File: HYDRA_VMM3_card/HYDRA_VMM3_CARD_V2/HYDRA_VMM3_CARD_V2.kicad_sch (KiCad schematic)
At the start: 17 parts, among them J1 ME1014010101011

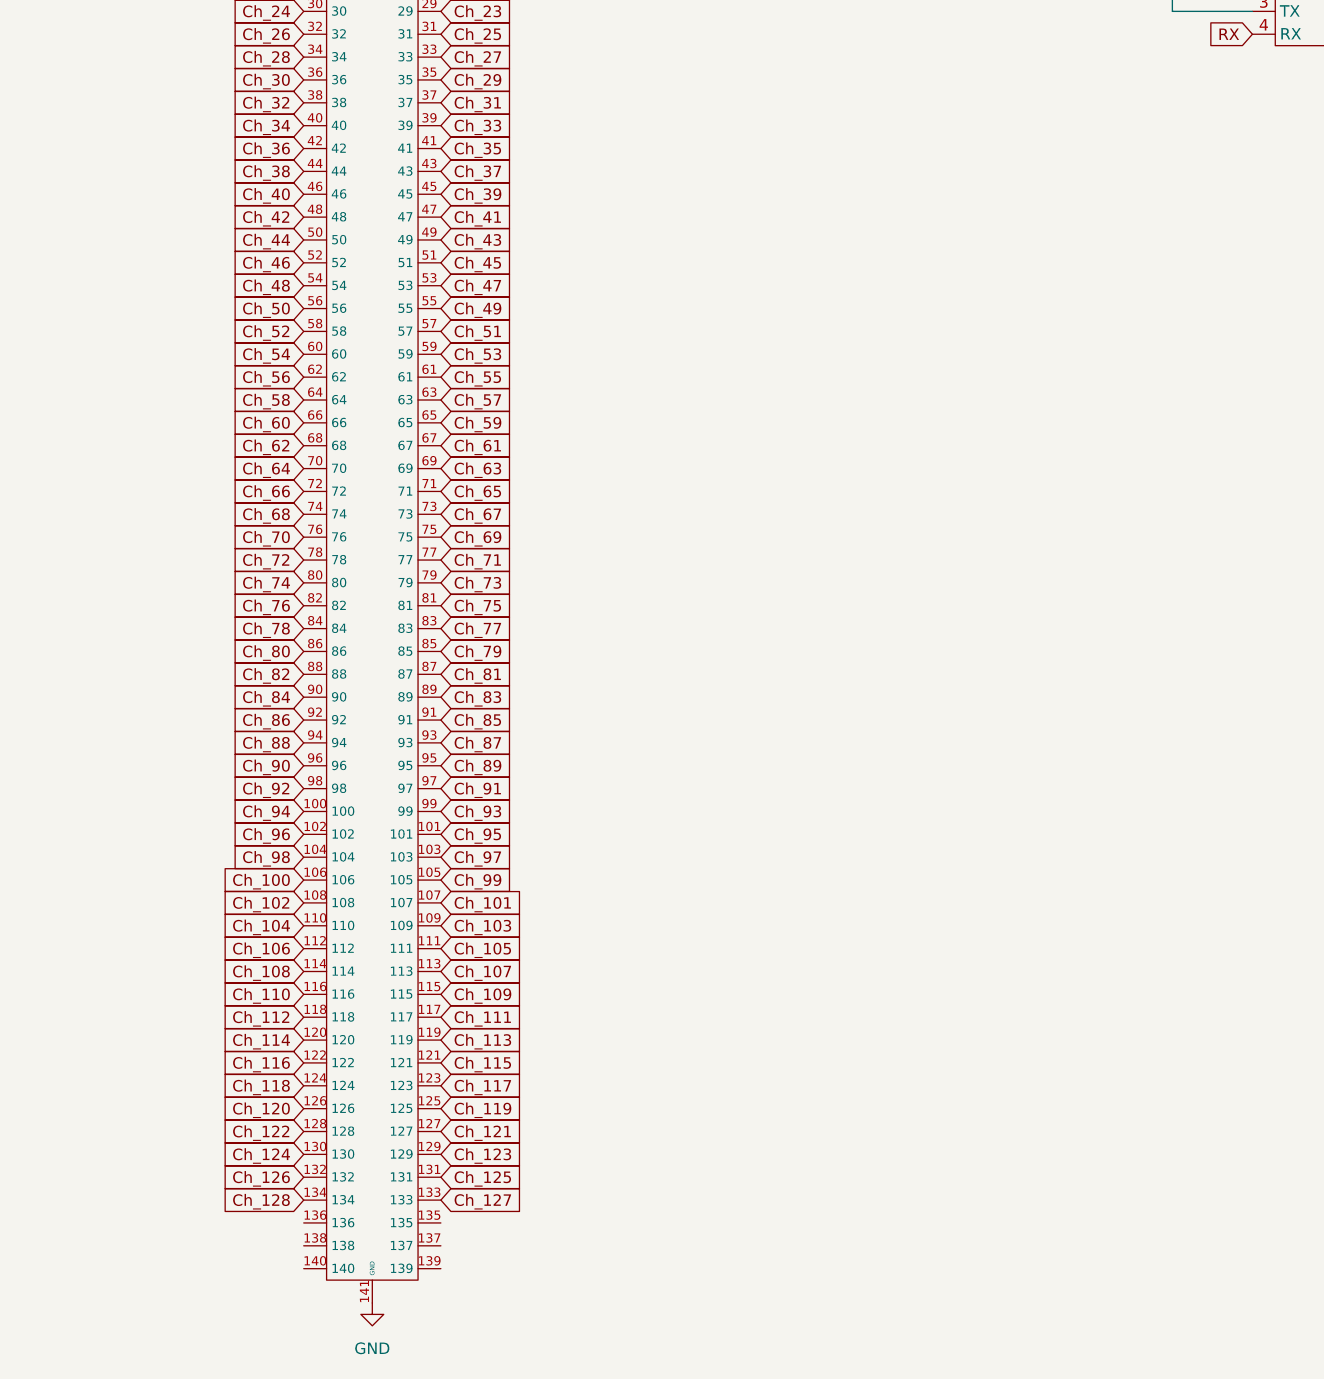
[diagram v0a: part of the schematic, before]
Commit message: .
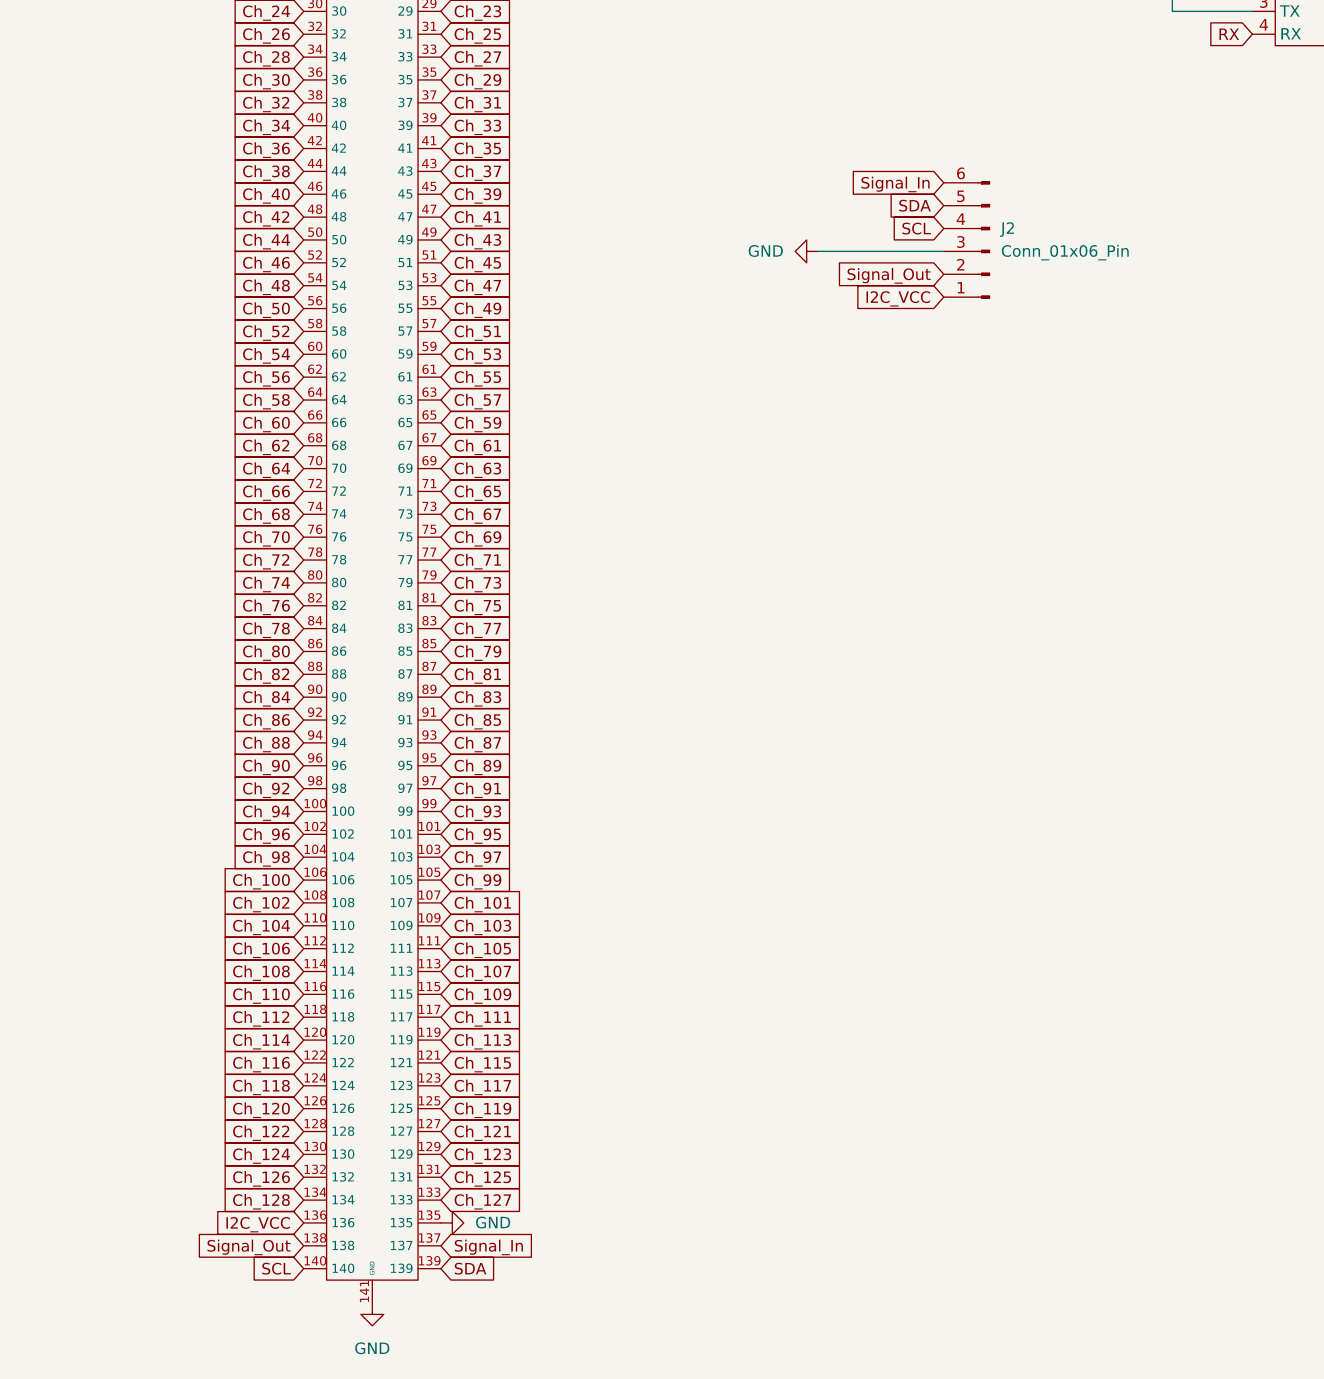
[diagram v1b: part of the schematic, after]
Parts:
- added J2: Conn_01x06_Pin, Connector_PinHeader_1.00mm:PinHeader_1x06_P1.00mm_Horizontal, symbol Connector:Conn_01x06_Pin
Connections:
- net GND: now also U1.135, J2.3 (Pin_3)
- net I2C_VCC: now reaches U1.136
- net I2C_VCC: now also J2.1 (Pin_1)
- net Signal_In: now reaches U1.137
- net Signal_In: now also J2.6 (Pin_6)
- net Signal_Out: now reaches U1.138
- net Signal_Out: now also J2.2 (Pin_2)
- net SDA: now reaches U1.139
- net SDA: now also J2.5 (Pin_5)
- net SCL: now reaches U1.140
- net SCL: now also J2.4 (Pin_4)

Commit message: .
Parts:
- removed J2: Conn_01x06_Pin, Connector_PinHeader_1.00mm:PinHeader_1x06_P1.00mm_Horizontal, symbol Connector:Conn_01x06_Pin
- removed Sig1, Sig2: 20449-001E-03, IPEX:IPEX_20449-001E-03, symbol IPEX:20449-001E-03
- removed Temp_2: ~, IPEX:TMP104, symbol IPEX:TMP104
- added R3, R4, R5, R6, R7, R8: 10k, Resistor_SMD:R_0201_0603Metric, symbol Device:R
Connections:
- net +1V8: now also J1.B1, J1.B2, J1.B3, J1.B4; no longer J1.A10, J1.A5, J1.A6, J1.A7, J1.A8, J1.A9
- net +3V3: now also J1.B10, J1.B8, J1.B9; no longer J1.B1, J1.B2, J1.B3, J1.B4
- net GND: now also J1.A5, J1.A7, J1.A8, J1.A9, R3.2, R4.2, R5.2, R6.2, R7.2, R8.2; no longer J1.B10, J1.B8, J1.B9, U1.135
- net RX: now also Temp_1.4 (RX)
- net bit_0: now reaches U1.1
- net bit_0: now also R3.1
- net bit_1: now reaches U1.2
- net bit_1: now also R4.1
- net bit_2: now reaches U1.3
- net bit_2: now also R5.1
- net bit_3: now reaches U1.4
- net bit_3: now also R8.1
- net bit_4: now reaches U1.5
- net bit_4: now also R7.1
- net bit_5: now reaches U1.6
- net bit_5: now also R6.1
- net I2C_VCC: no longer names the net of U1.136
- net SCL: no longer names the net of U1.140
- net SDA: no longer names the net of U1.139
- net Signal_In: no longer names the net of U1.137
- net Signal_Out: no longer names the net of U1.138
- new net Heimtime: J1.A10
- new net Master_Trigg: J1.A6
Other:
- note added: "6 bit geographical code"
- note added: "Power LEDs"
- note added: "Temperature Readout"
- moved on the sheet: 1.8V1, 1.8V_2.5A1, 1.8_On1, 3.3V1, 3.3V_0.5A1, 3.3V_On1, GND1, J1A, J1B, R1, R2, Temp_1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
